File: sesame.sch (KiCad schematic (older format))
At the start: 154 parts, among them U1 ATmega32A-PU

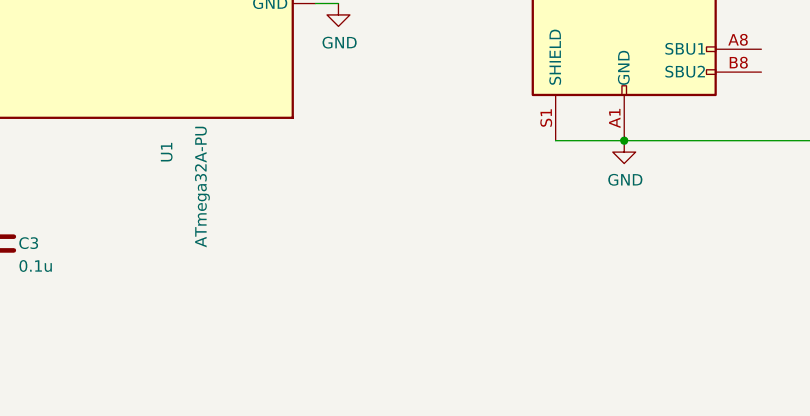
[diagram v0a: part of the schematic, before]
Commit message: minor design changes
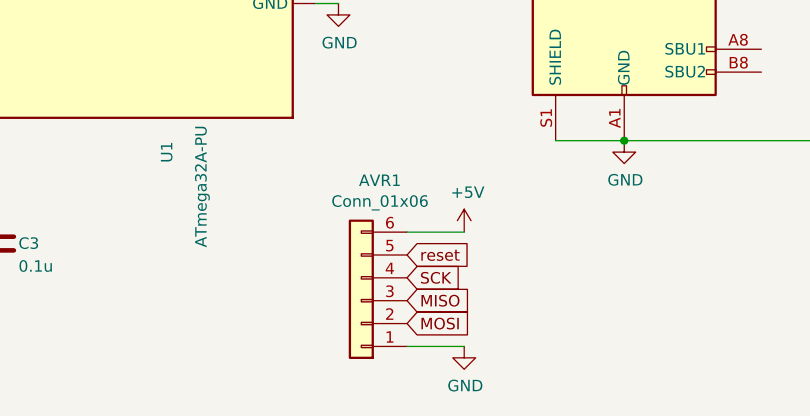
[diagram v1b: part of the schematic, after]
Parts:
- added AVR1: Conn_01x06, Connector_PinHeader_2.54mm:PinHeader_1x06_P2.54mm_Vertical, symbol Connector_Generic:Conn_01x06
- C1: footprint Capacitor_THT:CP_Radial_D5.0mm_P2.50mm -> Capacitor_THT:CP_Radial_D4.0mm_P1.50mm
- MX15: footprint MX_Only:MXOnly-2.25U-NoLED -> MX_Only:MXOnly-2U-NoLED
- MX31: footprint MX_Only:MXOnly-1U-NoLED -> MX_Only:MXOnly-1.5U-NoLED
- MX59: footprint MX_Only:MXOnly-1.5U-NoLED -> MX_Only:MXOnly-1.75U-NoLED
- MX61: footprint MX_Only:MXOnly-2.25U-NoLED -> MX_Only:MXOnly-2.75U-NoLED
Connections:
- net +5V: now also AVR1.6 (Pin_6)
- net GND: now also AVR1.1 (Pin_1)
- net MISO: now also AVR1.3 (Pin_3)
- net MOSI: now also AVR1.2 (Pin_2)
- net SCK: now also AVR1.4 (Pin_4)
- net reset: now also AVR1.5 (Pin_5)
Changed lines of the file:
@@
 F 0 "C1" H 3100 6850 50  0000 L CNN
 F 1 "4.7u" H 3100 6750 50  0000 L CNN
-F 2 "Capacitor_THT:CP_Radial_D5.0mm_P2.50mm" H 3000 6850 50  0001 C CNN
+F 2 "Capacitor_THT:CP_Radial_D4.0mm_P1.50mm" H 3000 6850 50  0001 C CNN
 F 3 "~" H 3000 6850 50  0001 C CNN
 	1    3000 6850
@@
 F 0 "MX15" H 9550 1100 60  0000 C CNN
 F 1 "MX-NoLED" H 9550 1050 20  0000 C CNN
-F 2 "MX_Only:MXOnly-2.25U-NoLED" H 8975 875 60  0001 C CNN
+F 2 "MX_Only:MXOnly-2U-NoLED" H 8975 875 60  0001 C CNN
 F 3 "" H 8975 875 60  0001 C CNN
 	1    9600 900
@@
 F 0 "MX31" H 9633 1873 60  0000 C CNN
 F 1 "MX-NoLED" H 9633 1799 20  0000 C CNN
-F 2 "MX_Only:MXOnly-1U-NoLED" H 8975 1625 60  0001 C CNN
+F 2 "MX_Only:MXOnly-1.5U-NoLED" H 8975 1625 60  0001 C CNN
 F 3 "" H 8975 1625 60  0001 C CNN
 	1    9600 1650
@@
 F 0 "MX59" H 9083 3373 60  0000 C CNN
 F 1 "MX-NoLED" H 9083 3299 20  0000 C CNN
-F 2 "MX_Only:MXOnly-1.5U-NoLED" H 8425 3125 60  0001 C CNN
+F 2 "MX_Only:MXOnly-1.75U-NoLED" H 8425 3125 60  0001 C CNN
 F 3 "" H 8425 3125 60  0001 C CNN
 	1    9050 3150
@@
 F 0 "MX61" H 10100 3350 60  0000 C CNN
 F 1 "MX-NoLED" H 10100 3300 20  0000 C CNN
-F 2 "MX_Only:MXOnly-2.25U-NoLED" H 9525 3125 60  0001 C CNN
+F 2 "MX_Only:MXOnly-2.75U-NoLED" H 9525 3125 60  0001 C CNN
 F 3 "" H 9525 3125 60  0001 C CNN
 	1    10150 3150
@@
 Text GLabel 1100 2550 0    50   Input ~ 0
 caps
+Text GLabel 5500 7200 2    50   Input ~ 0
+MOSI
+Text GLabel 5500 7100 2    50   Input ~ 0
+MISO
+Text GLabel 5500 7000 2    50   Input ~ 0
+SCK
+$Comp
+L power:GND #PWR0101
+U 1 1 5F329387
+P 5750 7300
+F 0 "#PWR0101" H 5750 7050 50  0001 C CNN
+F 1 "GND" H 5755 7127 50  0000 C CNN
+F 2 "" H 5750 7300 50  0001 C CNN
+F 3 "" H 5750 7300 50  0001 C CNN
+	1    5750 7300
+	1    0    0    -1
+$EndComp
+$Comp
+L power:+5V #PWR0102
+U 1 1 5F329944
+P 5750 6800
+F 0 "#PWR0102" H 5750 6650 50  0001 C CNN
+F 1 "+5V" H 5765 6973 50  0000 C CNN
+F 2 "" H 5750 6800 50  0001 C CNN
+F 3 "" H 5750 6800 50  0001 C CNN
+	1    5750 6800
+	1    0    0    -1
+$EndComp
+Text GLabel 5500 6900 2    50   Input ~ 0
+reset
+$Comp
+L Connector_Generic:Conn_01x06 AVR1
+U 1 1 5F32D9BD
+P 5300 7100
+F 0 "AVR1" H 5218 6575 50  0000 C CNN
+F 1 "Conn_01x06" H 5218 6666 50  0000 C CNN
+F 2 "Connector_PinHeader_2.54mm:PinHeader_1x06_P2.54mm_Vertical" H 5300 7100 50  0001 C CNN
+F 3 "~" H 5300 7100 50  0001 C CNN
+	1    5300 7100
+	-1   0    0    1
+$EndComp
+Wire Wire Line
+	5500 7300 5750 7300
+Wire Wire Line
+	5500 6800 5750 6800
 $EndSCHEMATC
